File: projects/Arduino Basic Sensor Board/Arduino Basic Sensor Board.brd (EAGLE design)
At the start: 68.6 x 53.3 mm, 56 parts, among them Q1 S8050SOT23, Q2 S8050SOT23, U1 74HC595N-DIP16

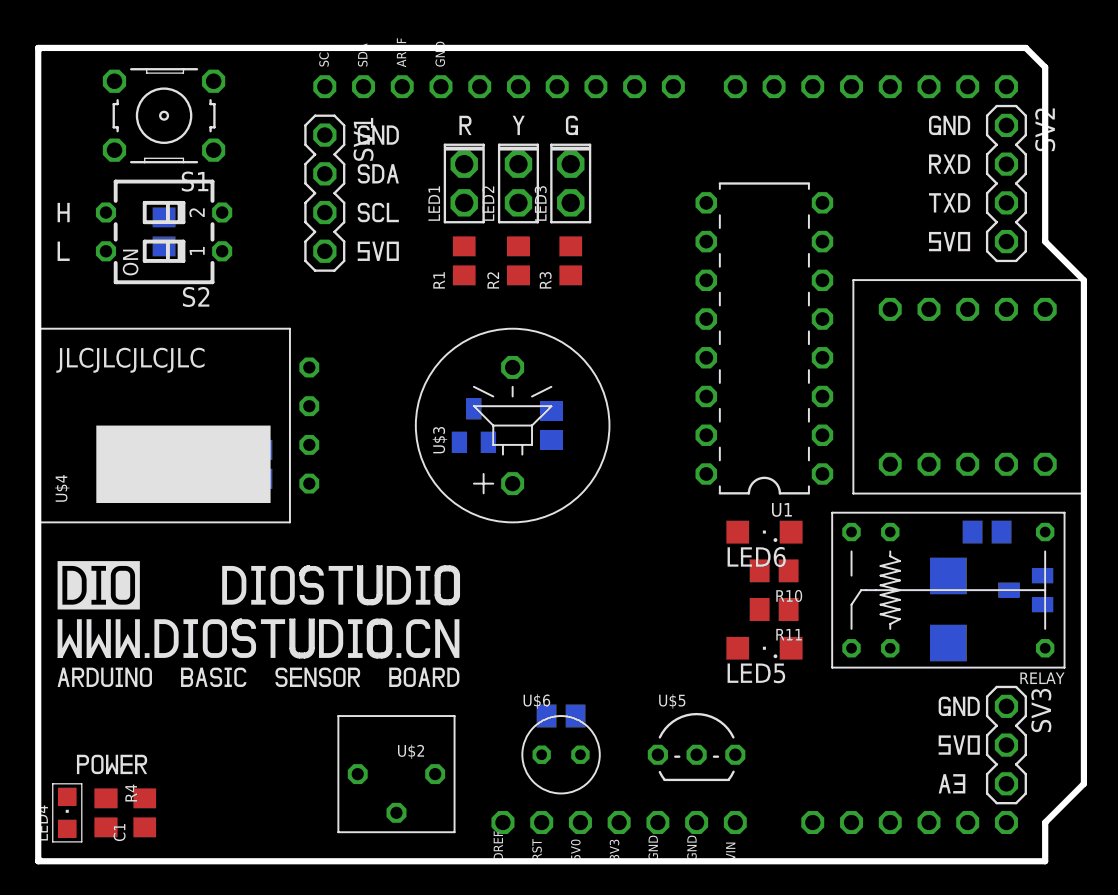
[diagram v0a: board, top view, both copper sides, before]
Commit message: 2020.06.08.01
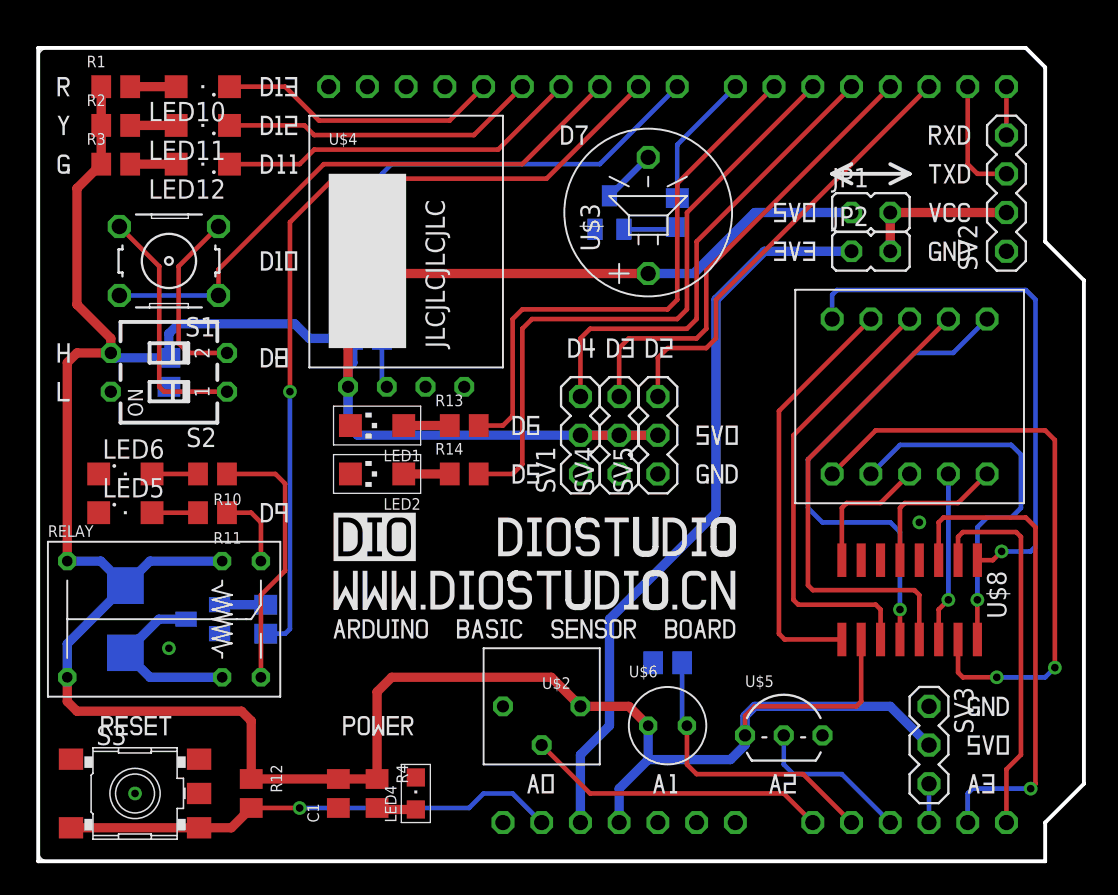
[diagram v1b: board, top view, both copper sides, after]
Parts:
- removed LED3: GREEN, Display:LED2X5
- removed U1: 74HC595N-DIP16, Chip:DIP16-2.54-20.32X5.84MM
- added JP1, JP2: (no value), Jumper:JP1Q
- added LED10: RED, Display:SML1206
- added LED11: YELLOW, Display:SML1206
- added LED12: GREEN, Display:SML1206
- added R12, R13, R14: 103, RCLDA:R0805
- added S3: TS-SMD_6S6_SHIELD, Button:TS-SMD_6*6_SHIELD
- added SV4, SV5: (no value), Pin-Header:MA03-1
- added U$11: (no value), Logos:D10_050
- added U$12: (no value), Logos:D13_050
- added U$31: (no value), Logos:D12_050
- added U$32: (no value), Logos:D6_050
- added U$33: (no value), Logos:D8_050
- added U$34: (no value), Logos:D9_050
- added U$35: (no value), Logos:D7_050
- added U$36: (no value), Logos:A0_050
- added U$37: (no value), Logos:A1_050
- added U$38: (no value), Logos:A2_050
- added U$39: (no value), Logos:MAKE_SOMETHING_FUN_050
- added U$40: (no value), Logos:5V0_050
- added U$41: (no value), Logos:GND_050
- added U$42: (no value), Logos:VCC_050
- added U$43: (no value), Logos:3V3_050
- added U$44: (no value), Logos:GREEN_050
- added U$45: (no value), Logos:RED_050
- added U$46: (no value), Logos:YELLOW_050
- LED1: value RED -> (none); device Display:LED2X5 -> Display:LED1206
- LED2: value YELLOW -> (none); device Display:LED2X5 -> Display:LED1206
- SV1: device Pin-Header:MA04-1 -> Pin-Header:MA03-1
- U$14: device Logos:RED_050 -> Logos:RESET_050
- U$15: value (none) -> 3261AS; device Logos:YELLOW_050 -> Display:TN_AS_2_0.36INCH
- U$16: device Logos:SCL_050 -> Logos:D4_050
- U$23: device Logos:SDA_050 -> Logos:D3_050
- U$24: device Logos:GND_050 -> Logos:D2_050
- U$25: device Logos:5V0_050 -> Logos:D5_050
- U$8: value LG3622BH -> TM1650; device Display:LG3622BH -> Chip:SO16
- U$9: device Logos:GREEN_050 -> Logos:D11_050
- moved Q1 54.0 mm to (-0.64, -51.4)
- moved D1 54.0 mm to (-5.71, -51.4), turned to 270 degrees
- moved RELAY 51.5 mm to (-3.17, -51.4), turned to 0 degrees
- moved R7 47.7 mm to (3.49, -51.4), turned to 90 degrees
- moved U$14 45.8 mm to (-7.30, -59.1)
- moved LED5 42.8 mm to (-5.71, -44.5), turned to 0 degrees
- moved LED6 42.1 mm to (-5.71, -41.9), turned to 0 degrees
- moved R10 37.4 mm to (0.00, -41.9)
- moved R11 37.4 mm to (0.00, -44.5)
- moved U$15 31.2 mm to (45.7, -36.8)
- moved R3 30.5 mm to (-6.35, -21.6), turned to 0 degrees
- moved R2 27.9 mm to (-6.35, -19.1), turned to 0 degrees
- moved R1 25.6 mm to (-6.35, -16.5), turned to 0 degrees
- moved U$24 23.5 mm to (28.4, -34.3)
- moved SV1 23.1 mm to (24.1, -39.4), turned to 90 degrees
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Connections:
- removed net A4: U$1.A4
- removed net A5: U$1.A5
- new net DIG1: U$15.10, U$8.1
- new net DIG2: U$15.5, U$8.5
- new net N$12: LED2.A, R14.1
- new net N$13: JP1.2, JP2.2, SV2.2
- new net N$7: LED1.A, R13.1
- net 3V3: now also JP2.1
- net 5V0: now also JP1.1, R12.1, SV1.2, SV4.2, SV5.2, U$8.10; no longer SV1.4, SV2.4, U1.10, U1.16
- net A: now also U$15.3, U$8.8; no longer U$8.A, U1.15
- net B: now also U$15.9, U$8.9; no longer U$8.B, U1.1
- net C: now also U$15.8, U$8.11; no longer U$8.C, U1.2
- net D: now also U$15.6, U$8.12; no longer U$8.D, U1.3
- net D11: now also LED12.C; no longer LED3.K
- net D12: now also LED11.C; no longer LED2.K
- net D13: now also LED10.C; no longer LED1.K
- net D2: now also SV5.3; no longer U$8.2
- net D3: now also SV4.3; no longer U$8.1
- net D4: now also SV1.3; no longer U1.12
- net D5: now also R14.2; no longer U1.11
- net D6: now also R13.2; no longer U1.14
- net D7: now also R8.1; no longer R9.2, U$4.DAT
- net D8: now also R9.2, U$4.DAT; no longer R8.1
- net E: now also U$15.7, U$8.13; no longer U$8.E, U1.4
- net F: now also U$15.4, U$8.14; no longer U$8.F, U1.5
- net G: now also U$15.1, U$8.15; no longer U$8.G, U1.6
- net GND: now also LED1.C, LED2.C, S3.1, S3.2, S3.5, SV4.1, SV5.1, U$8.4; no longer U1.13, U1.8
- net H: now also U$15.2, U$8.16; no longer U$8.H, U1.7
- net N$1: now also LED10.A; no longer LED1.A
- net N$2: now also LED11.A; no longer LED2.A
- net N$3: now also LED12.A; no longer LED3.A
- net RESET: now also R12.2, S3.3, S3.4
- net RXD: now also SV2.4; no longer SV2.2
- net SCL: now also U$1.A5, U$8.2; no longer SV1.3, U$1.SCL
- net SDA: now also U$1.A4, U$8.3; no longer SV1.2, U$1.SDA
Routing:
- net 5V0: track 0.00 -> 239.7 mm
- net D9: track 0.00 -> 54.9 mm, vias 0 -> 1
- net 3V3: track 0.00 -> 48.2 mm
- net D5: track 0.00 -> 41.4 mm
- net G: track 0.00 -> 39.9 mm, vias 0 -> 2
- net D10: track 0.00 -> 38.2 mm
- net D6: track 0.00 -> 36.8 mm
- net D8: track 0.00 -> 35.8 mm
- net DIG1: track 0.00 -> 35.7 mm, vias 0 -> 1
- net SDA: track 0.00 -> 32.7 mm, vias 0 -> 1
- net RESET: track 0.00 -> 32.6 mm, vias 0 -> 1
- net D: track 0.00 -> 32.5 mm, vias 0 -> 1
- net E: track 0.00 -> 31.8 mm
- net D4: track 0.00 -> 31.4 mm
- net D3: track 0.00 -> 30.3 mm
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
